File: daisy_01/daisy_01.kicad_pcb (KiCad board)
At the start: 2 copper layers, 106.7 x 30.5 mm, 17 parts, among them J1 AudioInput, J2 AudioOutput1, J3 AudioOutput2, Q1 PN2222A, SW1 SW_SPST, SW2 RotaryEncoder_Switch

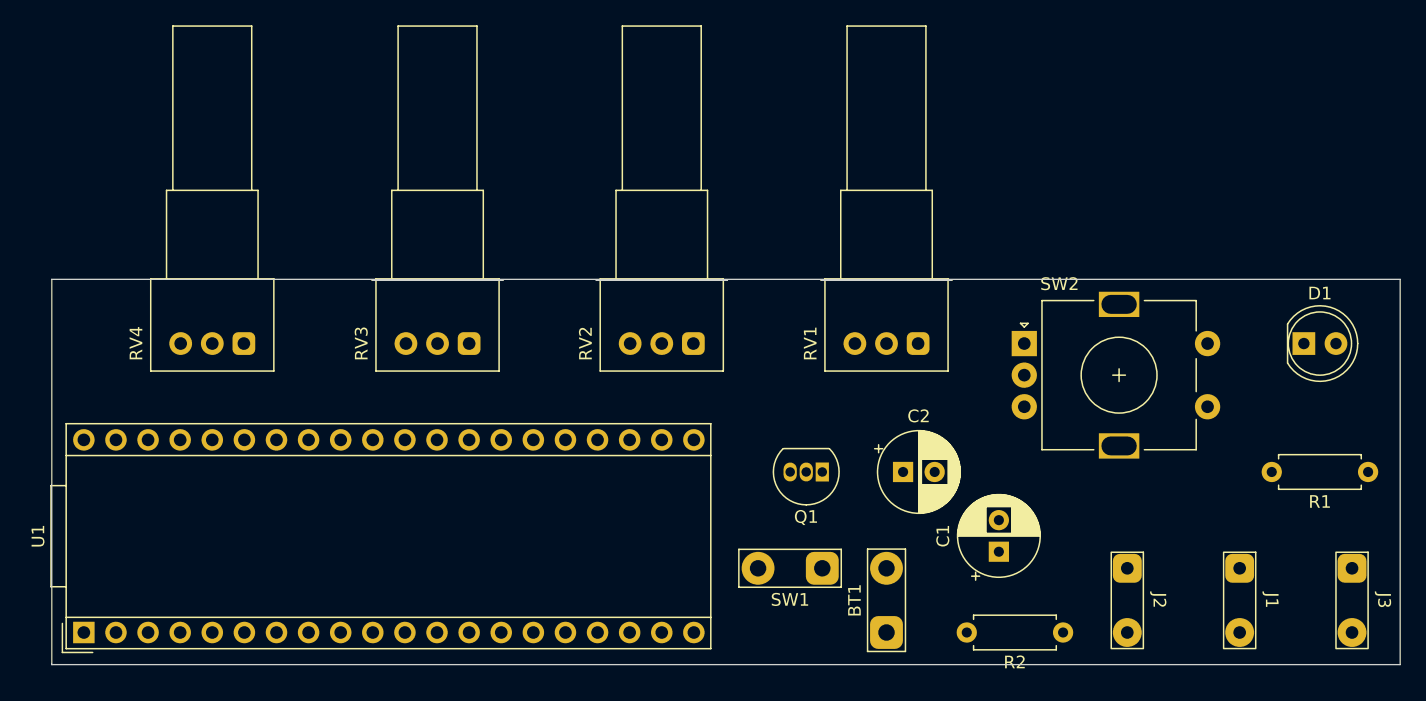
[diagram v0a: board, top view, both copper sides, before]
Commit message: update
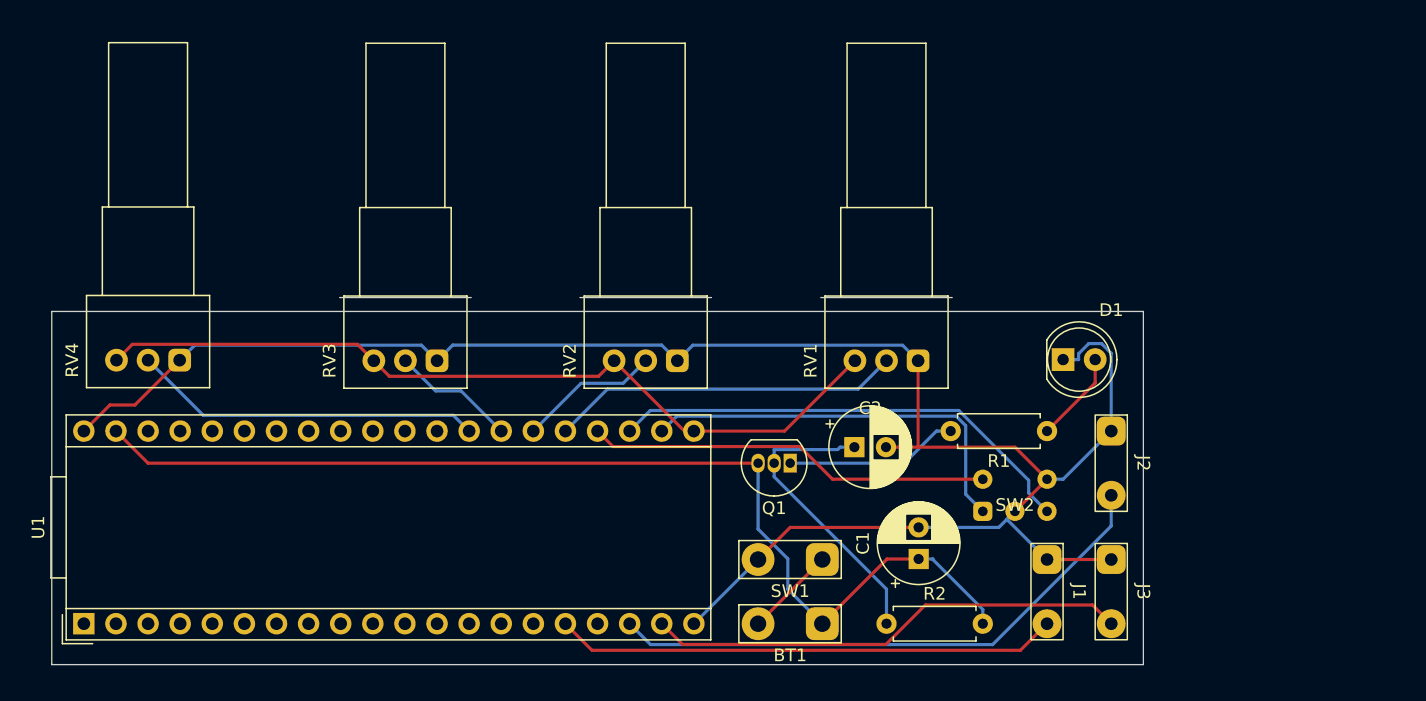
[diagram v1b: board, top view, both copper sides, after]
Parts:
- SW2: footprint Rotary_Encoder:RotaryEncoder_Alps_EC11E-Switch_Vertical_H20mm -> personal_footprints:ec11_encoder_mio
- moved R1 25.6 mm to (180.3, 113.6)
- moved D1 19.1 mm to (181.6, 108.0)
- moved J3 19.1 mm to (185.4, 126.3)
- moved J1 15.3 mm to (180.3, 126.3)
- moved R2 14.0 mm to (167.6, 128.8), turned to 0 degrees
- moved SW2 13.3 mm to (177.8, 120.0)
- moved J2 10.9 mm to (185.4, 116.1)
- moved C1 6.38 mm to (170.2, 123.7)
- moved RV4 5.25 mm to (111.7, 108.0)
- moved BT1 5.13 mm to (162.6, 128.8), turned to 180 degrees
- moved C2 4.32 mm to (165.1, 114.9)
- moved RV3 2.88 mm to (132.1, 108.0)
- moved Q1 2.63 mm to (160.0, 116.1)
- moved RV2 1.86 mm to (151.1, 108.0)
- moved RV1 1.36 mm to (170.1, 108.0)
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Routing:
- net GND: track 0.00 -> 152.0 mm
- net +9V: track 0.00 -> 84.3 mm
- net /A_PWR3.3: track 0.00 -> 65.1 mm
- net Net-(U1-Audio_Out_1): track 0.00 -> 45.1 mm
- net Net-(J1-PadT): track 0.00 -> 39.8 mm
- net Net-(U1-Audio_Out_2): track 0.00 -> 38.1 mm
- net Net-(U1-A1/D16): track 0.00 -> 37.6 mm
- net Net-(U1-A0/D15): track 0.00 -> 32.2 mm
- net Net-(U1-A2/D17): track 0.00 -> 32.1 mm
- net Net-(U1-A5/D21): track 0.00 -> 27.7 mm
- net Net-(U1-A3/D18): track 0.00 -> 27.7 mm
- net Net-(Q1-B): track 0.00 -> 23.9 mm
- net Net-(Q1-E): track 0.00 -> 13.8 mm
- net Net-(U1-A4/D19): track 0.00 -> 11.2 mm
- net Net-(U1-A5/D20): track 0.00 -> 9.88 mm
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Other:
- board size 106.7 x 30.5 mm -> 86.4 x 27.9 mm

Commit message: update gerber && drill
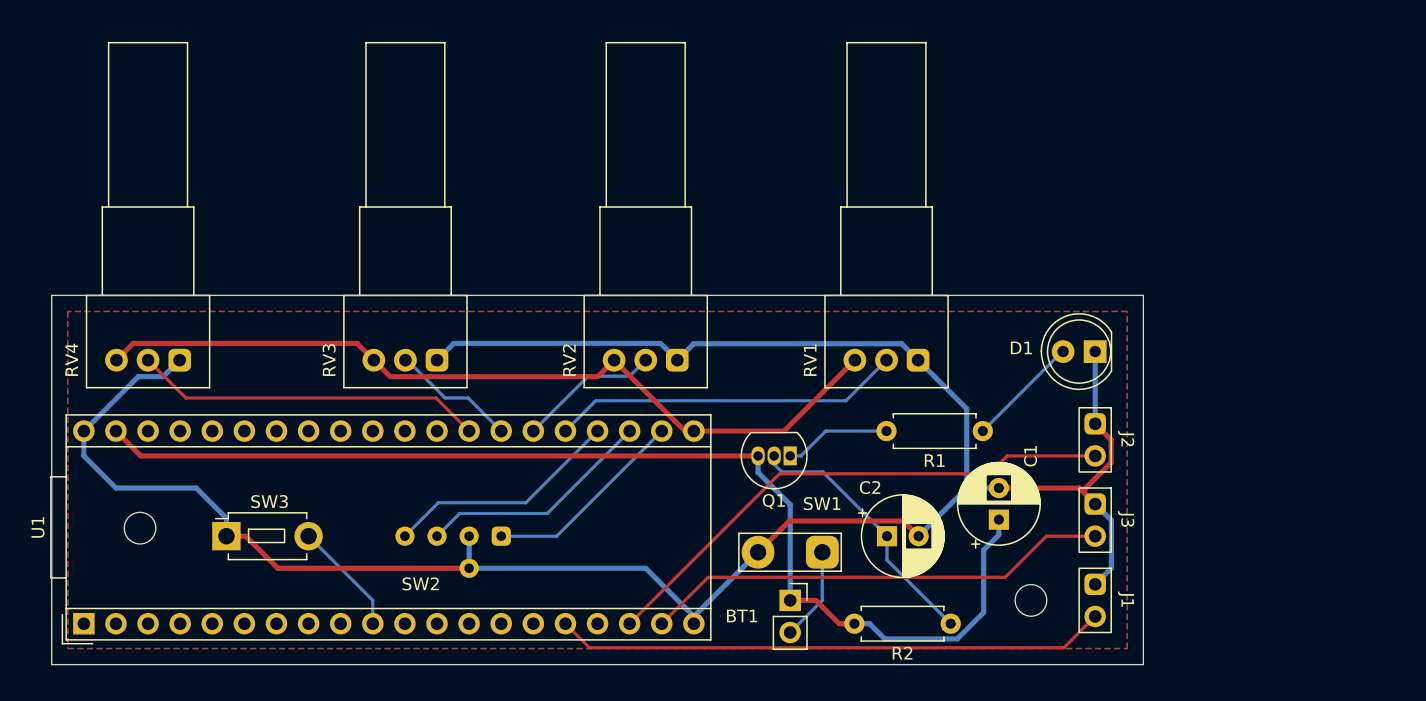
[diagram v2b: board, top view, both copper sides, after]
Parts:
- added SW3: SW_Push, Button_Switch_THT:SW_PUSH_1P1T_6x3.5mm_H5.0_APEM_MJTP1250, F.Cu at (115.4, 121.9)
- added screw1: MountingHole_2.5mm, MountingHole:MountingHole_2.5mm, F.Cu at (108.6, 121.3)
- added screw2: MountingHole_2.5mm, MountingHole:MountingHole_2.5mm, F.Cu at (179.1, 127.0)
- BT1: footprint TestPoint:TestPoint_2Pads_Pitch5.08mm_Drill1.3mm -> Connector_PinSocket_2.54mm:PinSocket_1x02_P2.54mm_Vertical
- moved SW2 43.2 mm to (134.6, 121.9), turned to 180 degrees
- moved C2 7.50 mm to (167.7, 121.9)
- moved C1 7.07 mm to (176.5, 120.6)
- moved R1 5.08 mm to (175.3, 113.6)
- moved R2 5.08 mm to (172.7, 128.8), turned to 180 degrees
- moved J3 4.56 mm to (184.2, 121.9)
- moved J1 4.29 mm to (184.2, 128.3)
- moved BT1 3.14 mm to (160.0, 127.0), turned to 0 degrees
- moved D1 2.62 mm to (184.2, 107.3), turned to 180 degrees
- moved J2 1.39 mm to (184.2, 115.6)
- moved Q1 0.57 mm to (160.0, 115.6)
- moved SW1 0.57 mm to (162.6, 123.2)
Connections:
- U1 pad 10: unconnected-(U1-D9-Pad10) -> Net-(U1-D9)
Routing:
- net GND: track 152.0 -> 178.7 mm
- net Net-(U1-A1/D16): track 37.6 -> 18.7 mm
- net Net-(U1-A0/D15): track 32.2 -> 16.1 mm
- net Net-(U1-A2/D17): track 32.1 -> 18.7 mm
- net Net-(U1-D9): track 0.00 -> 9.03 mm
- net Net-(Q1-E): track 13.8 -> 8.43 mm
- net +9V: track 84.3 -> 89.4 mm
- net Net-(J1-PadT): track 39.8 -> 43.7 mm
- net Net-(Q1-B): track 23.9 -> 21.0 mm
- net Net-(U1-Audio_Out_1): track 45.1 -> 42.3 mm
- net Net-(D1-A): track 7.23 -> 9.55 mm
- net Net-(U1-Audio_Out_2): track 38.1 -> 37.2 mm
- added copper zone on B.Cu, net GND
- added copper zone on F.Cu, net GND
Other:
- board size 86.4 x 27.9 mm -> 86.4 x 29.2 mm
- board text added: "neum pedal v1.0 2024.01"
